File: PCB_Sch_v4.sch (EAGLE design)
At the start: 51 parts, among them IC1 CP2104, M1 C0720B001F, Q1 MMBT2222LT1G, Q2 mmbt2222, Q3 DMG3415U, Q4 mmbt2222, SW1 2-1825027-0, SW2 2-1825027-0, SW3 2-1825027-0, SW4 2-1825027-0, SW5 2-1825027-0, U1 ESP32-WROOM-32D, U2 UG-2828GDEDF11, U3 MCP73831T-2ACI/OT, U4 AP2112-3.3, U5 FAN5331SX, X1 JSTPH, X4 20329

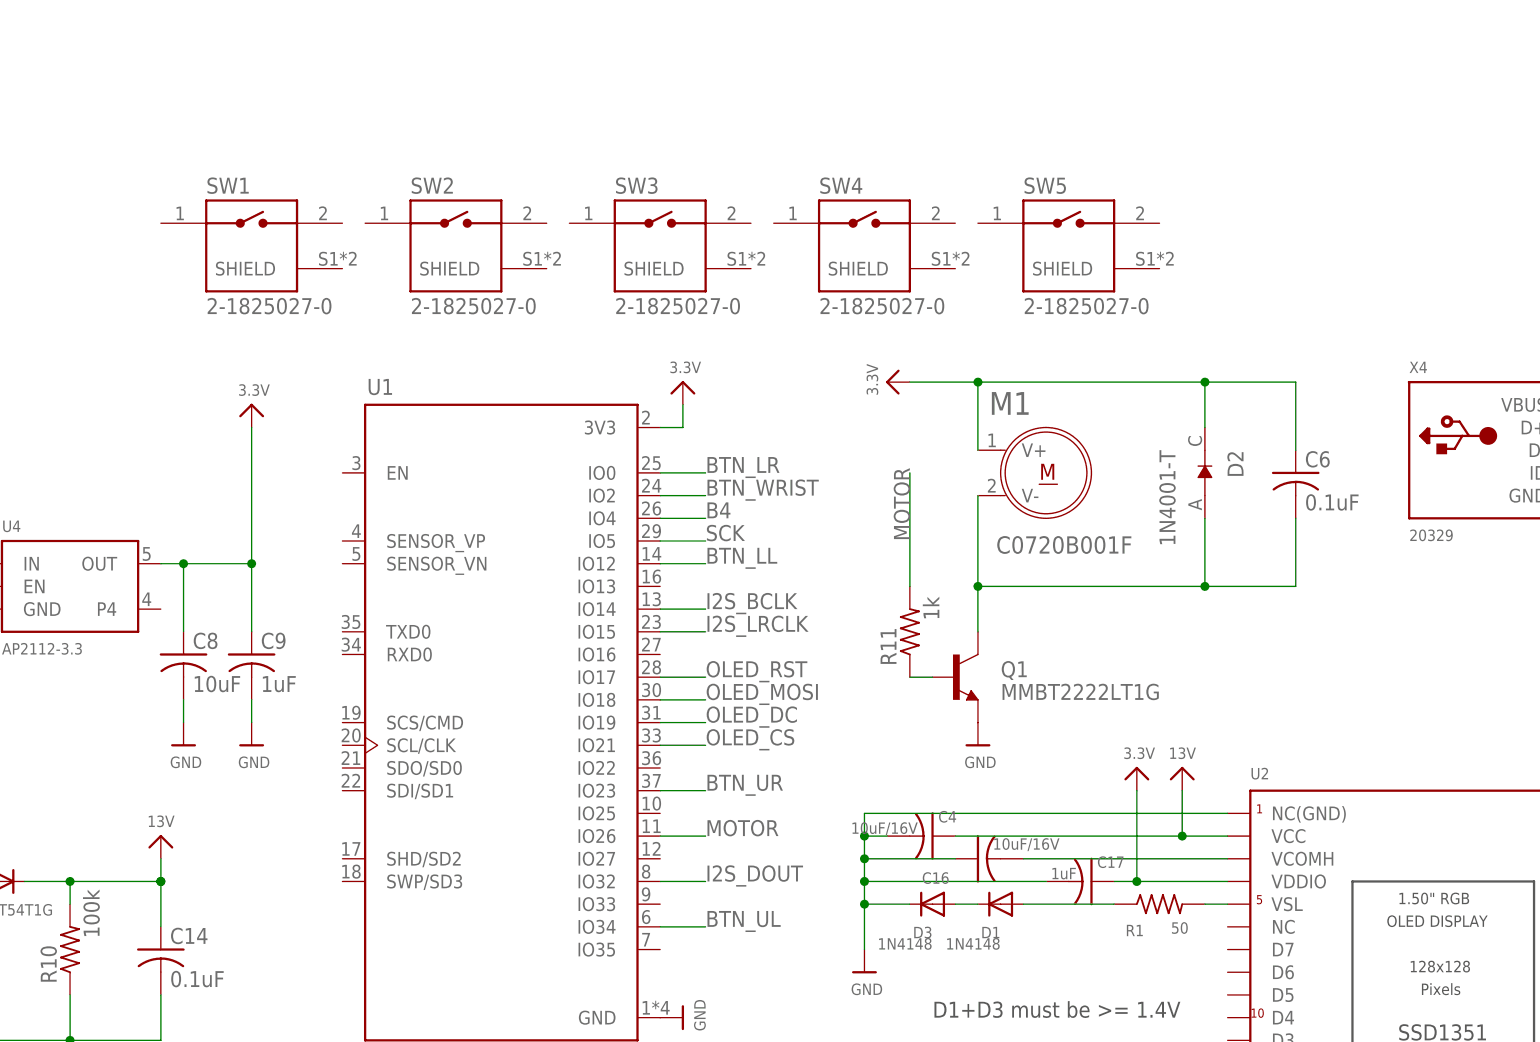
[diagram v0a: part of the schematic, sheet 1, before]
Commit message: Add files via upload
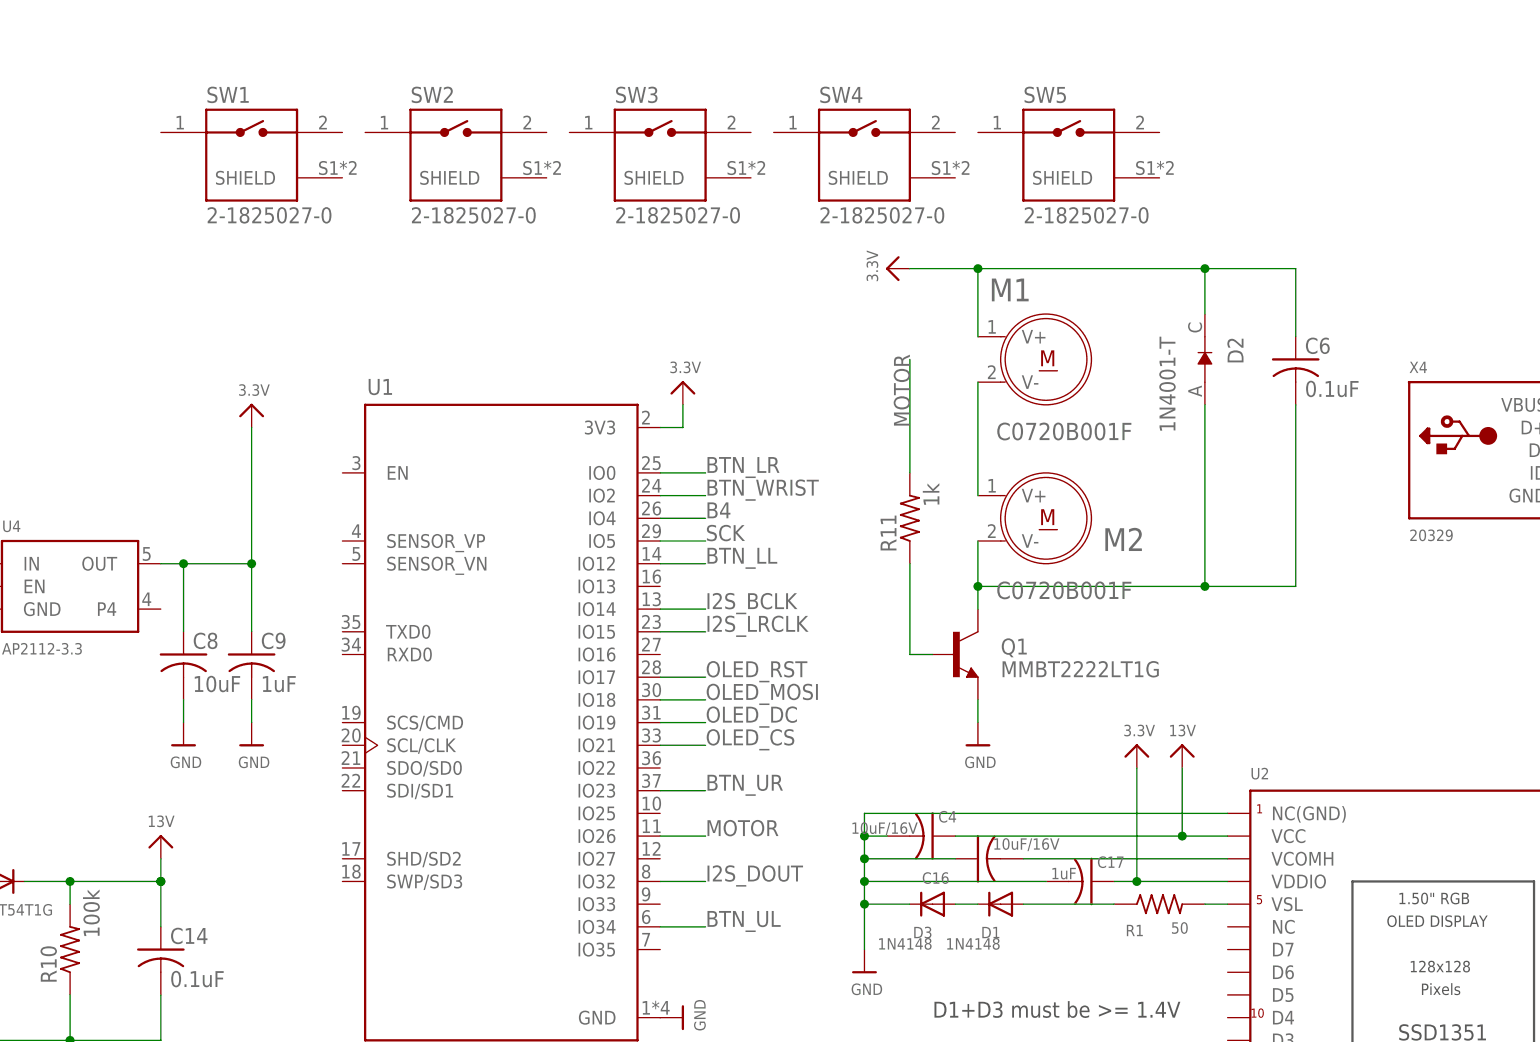
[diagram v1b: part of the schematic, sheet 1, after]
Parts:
- added M2: C0720B001F, C0720B001F:C0720B001F
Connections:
- new net N$20: M1.V-, M2.V+
- net N$4: now also M2.V-; no longer M1.V-
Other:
- moved on the sheet: C6, D2, M1, Q1, R11, SW1, SW2, SW3, SW4, SW5
